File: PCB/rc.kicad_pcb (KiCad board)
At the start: 2 copper layers, 54.9 x 25.4 mm, 8 parts, among them J1 USB_C_Receptacle_USB2.0_16P, J2 USB_A, J3 OLED display, U1 ESP32-S3-WROOM-1U, U2 MAX3421EEHJ+T, U3 ME6211C33M5

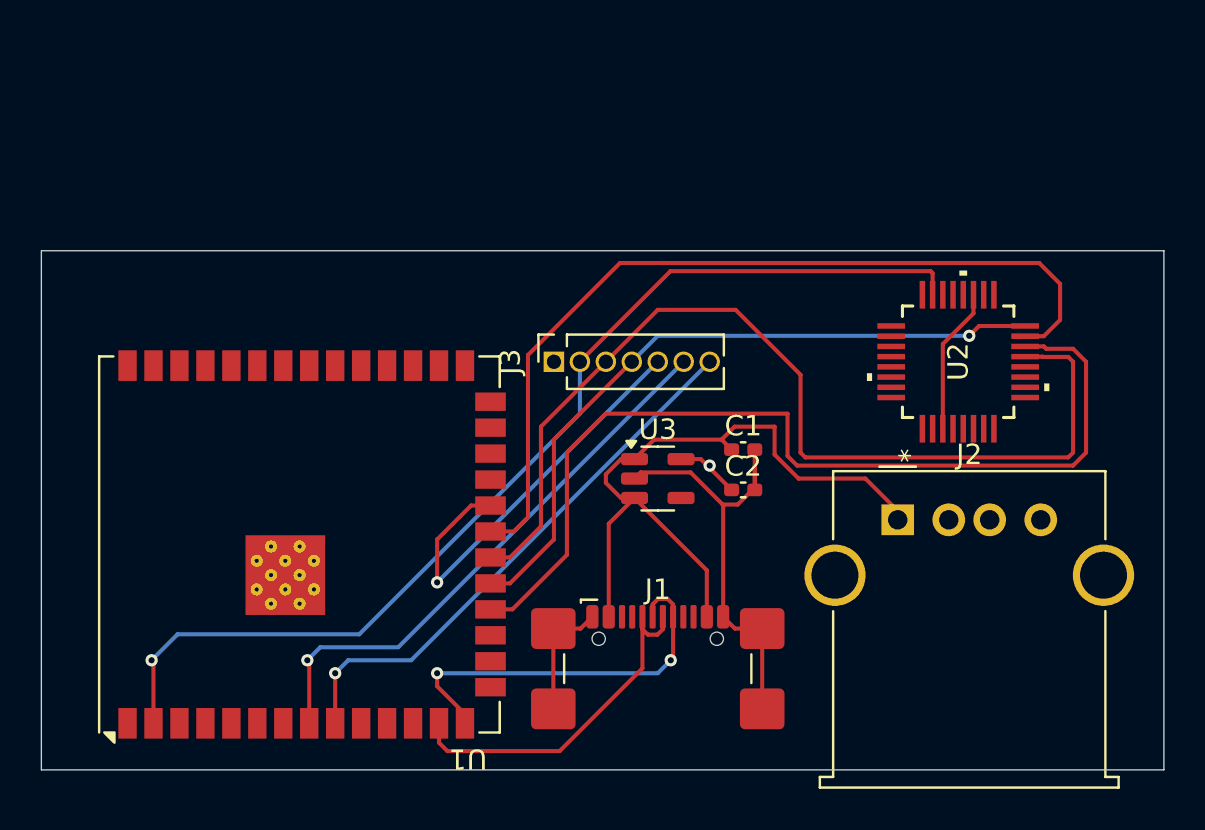
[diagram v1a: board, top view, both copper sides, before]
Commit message: pcb update
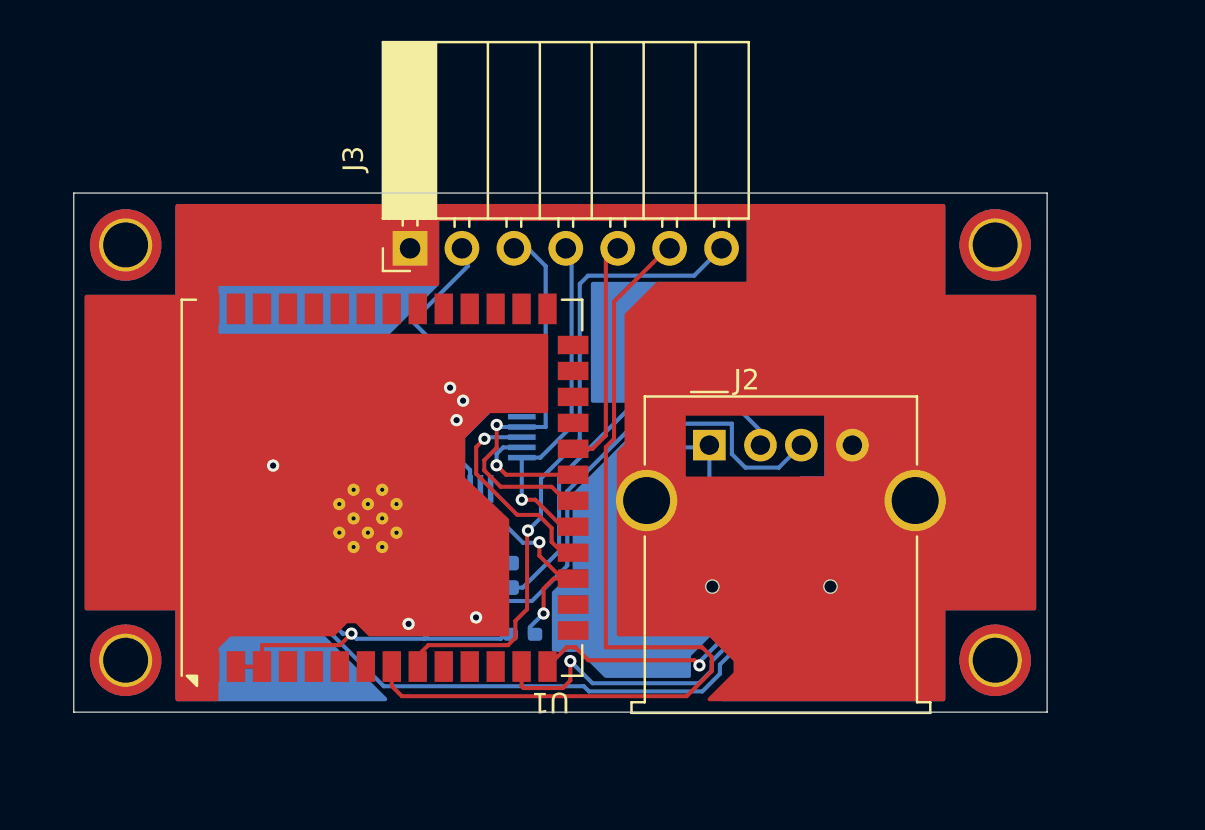
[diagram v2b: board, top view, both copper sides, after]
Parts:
- added C3: C, Capacitor_SMD:C_0402_1005Metric_Pad0.74x0.62mm_HandSolder, B.Cu at (40.1, 69.1)
- added C4: C, Capacitor_SMD:C_0402_1005Metric_Pad0.74x0.62mm_HandSolder, B.Cu at (44.2, 71.9)
- added C5: C, Capacitor_SMD:C_0402_1005Metric_Pad0.74x0.62mm_HandSolder, B.Cu at (57.4, 63.2)
- added C7: C, Capacitor_SMD:C_0402_1005Metric_Pad0.74x0.62mm_HandSolder, B.Cu at (46.5, 71.4)
- added D1: ESD9B5.0ST5G, Diode_SMD:D_SOD-923, B.Cu at (48.0, 68.5)
- added D2: ESD9B5.0ST5G, Diode_SMD:D_SOD-923, B.Cu at (49.0, 68.5)
- added FB1: FerriteBead, Inductor_SMD:L_0603_1608Metric, B.Cu at (48.5, 70.8)
- added FB2: FerriteBead, Inductor_SMD:L_0603_1608Metric, B.Cu at (61.7, 66.0)
- added R1: R_US, Resistor_SMD:R_0402_1005Metric_Pad0.72x0.64mm_HandSolder, B.Cu at (50.0, 69.5)
- added R2: R_US, Resistor_SMD:R_0402_1005Metric_Pad0.72x0.64mm_HandSolder, B.Cu at (47.0, 69.1)
- added R3: R_US, Resistor_SMD:R_0402_1005Metric_Pad0.72x0.64mm_HandSolder, B.Cu at (50.5, 72.4)
- added REF**: MountingHole_2.2mm_M2_ISO7380_Pad_TopBottom, MountingHole:MountingHole_2.2mm_M2_ISO7380_Pad_TopBottom, F.Cu at (73.7, 53.3)
- added REF**: MountingHole_2.2mm_M2_ISO7380_Pad_TopBottom, MountingHole:MountingHole_2.2mm_M2_ISO7380_Pad_TopBottom, F.Cu at (31.1, 73.7)
- added REF**: MountingHole_2.2mm_M2_ISO7380_Pad_TopBottom, MountingHole:MountingHole_2.2mm_M2_ISO7380_Pad_TopBottom, F.Cu at (31.1, 53.3)
- added REF**: MountingHole_2.2mm_M2_ISO7380_Pad_TopBottom, MountingHole:MountingHole_2.2mm_M2_ISO7380_Pad_TopBottom, F.Cu at (73.7, 73.7)
- added Y1: Crystal, Crystal:Crystal_SMD_G8-2Pin_3.2x1.5mm, B.Cu at (42.7, 70.1)
- C1, C2, J1, U2, U3: moved to B.Cu
- J3: footprint Connector_PinSocket_1.27mm:PinSocket_1x07_P1.27mm_Vertical -> Connector_PinSocket_2.54mm:PinSocket_1x07_P2.54mm_Horizontal
- moved U2 24.8 mm to (47.2, 62.0), turned to -90 degrees
- moved C2 24.3 mm to (37.1, 65.4), turned to -90 degrees
- moved C1 22.5 mm to (39.0, 65.4), turned to -90 degrees
- moved U3 20.1 mm to (37.4, 61.2), turned to -90 degrees
- moved J3 11.4 mm to (44.7, 53.1), turned to 90 degrees
- moved J2 9.91 mm to (59.7, 63.1)
- moved J1 6.12 mm to (62.7, 72.7), turned to 180 degrees
- moved U1 4.90 mm to (43.7, 65.2)
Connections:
- C1 pad 1: Net-(J2-VBUS) -> Net-(U3-CE)
- J1 pad A4: Net-(J2-VBUS) -> Net-(U3-CE)
- J1 pad A9: Net-(J2-VBUS) -> Net-(U3-CE)
- J1 pad B4: Net-(J2-VBUS) -> Net-(U3-CE)
- J1 pad B9: Net-(J2-VBUS) -> Net-(U3-CE)
- J2 pad 2: unconnected-(J2-D--Pad2) -> Net-(J2-D-)
- J2 pad 3: unconnected-(J2-D+-Pad3) -> Net-(J2-D+)
- U1 pad 17: unconnected-(U1-IO9-Pad17) -> Net-(U1-IO9)
- U1 pad 3: unconnected-(U1-EN-Pad3) -> Net-(J3-Pin_2)
- U2 pad 18: unconnected-(U2-INT-Pad18) -> Net-(U1-IO9)
- U2 pad 2: unconnected-(U2-VL-Pad2) -> Net-(J3-Pin_2)
- U2 pad 20: unconnected-(U2-D--Pad20) -> Net-(D2-A1)
- U2 pad 21: unconnected-(U2-D+-Pad21) -> Net-(D1-A1)
- U2 pad 22: unconnected-(U2-VBCOMP-Pad22) -> Net-(U2-VBCOMP)
- U2 pad 24: unconnected-(U2-XI-Pad24) -> Net-(U2-XI)
- U2 pad 25: unconnected-(U2-XO-Pad25) -> Net-(U2-XO)
- U3 pad 1: Net-(J2-VBUS) -> Net-(U3-CE)
- U3 pad 3: Net-(J2-VBUS) -> Net-(U3-CE)
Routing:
- net Net-(U3-CE): track 0.00 -> 60.4 mm
- net Net-(U1-IO13): track 42.2 -> 5.86 mm, vias 0 -> 1
- net Net-(U1-IO10): track 46.3 -> 10.5 mm, vias 0 -> 1
- net Net-(J2-VBUS): track 34.6 -> 5.20 mm
- net Net-(J3-Pin_3): track 48.6 -> 19.5 mm, vias 0 -> 1
- net Net-(J2-D+): track 0.00 -> 25.6 mm
- net Net-(J2-D-): track 0.00 -> 18.9 mm
- net Net-(J3-Pin_6): track 27.6 -> 44.8 mm, vias 1 -> 0
- net Net-(J3-Pin_4): track 34.2 -> 17.3 mm
- net Net-(J1-SHIELD): track 34.9 -> 20.2 mm, vias 0 -> 6
- net Net-(U1-IO9): track 0.00 -> 11.5 mm, vias 0 -> 2
- net Net-(U2-XO): track 0.00 -> 10.5 mm
- net Net-(J3-Pin_5): track 20.7 -> 11.3 mm, vias 1 -> 0
- net Net-(U2-XI): track 0.00 -> 7.12 mm
- net Net-(J3-Pin_2): track 55.0 -> 49.1 mm, vias 2 -> 1
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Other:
- board size 54.9 x 25.4 mm -> 47.6 x 25.4 mm
